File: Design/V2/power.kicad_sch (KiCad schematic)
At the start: 46 parts, among them U1 STM32H747BIT6

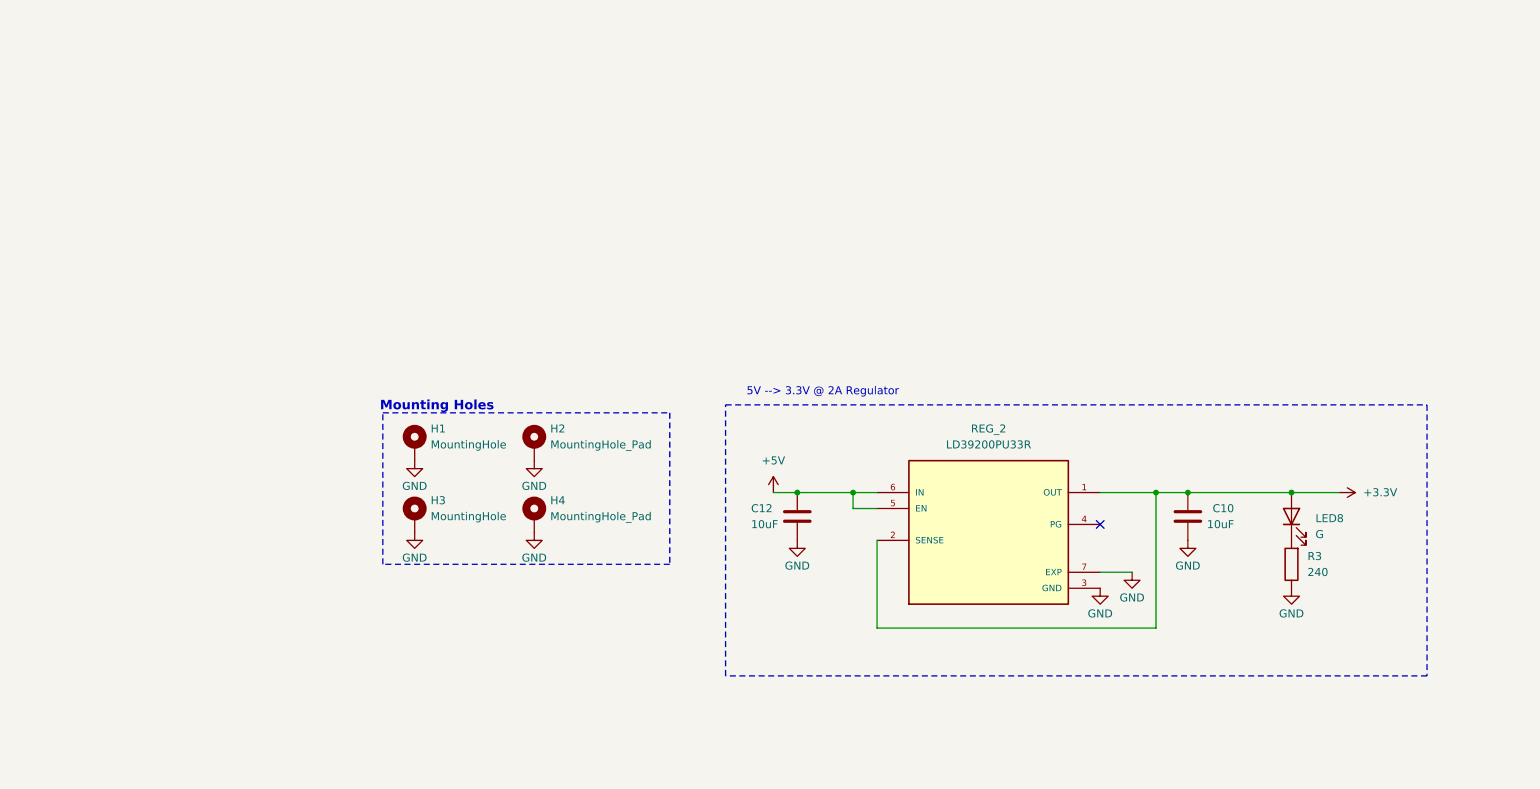
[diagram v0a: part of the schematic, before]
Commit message: power board
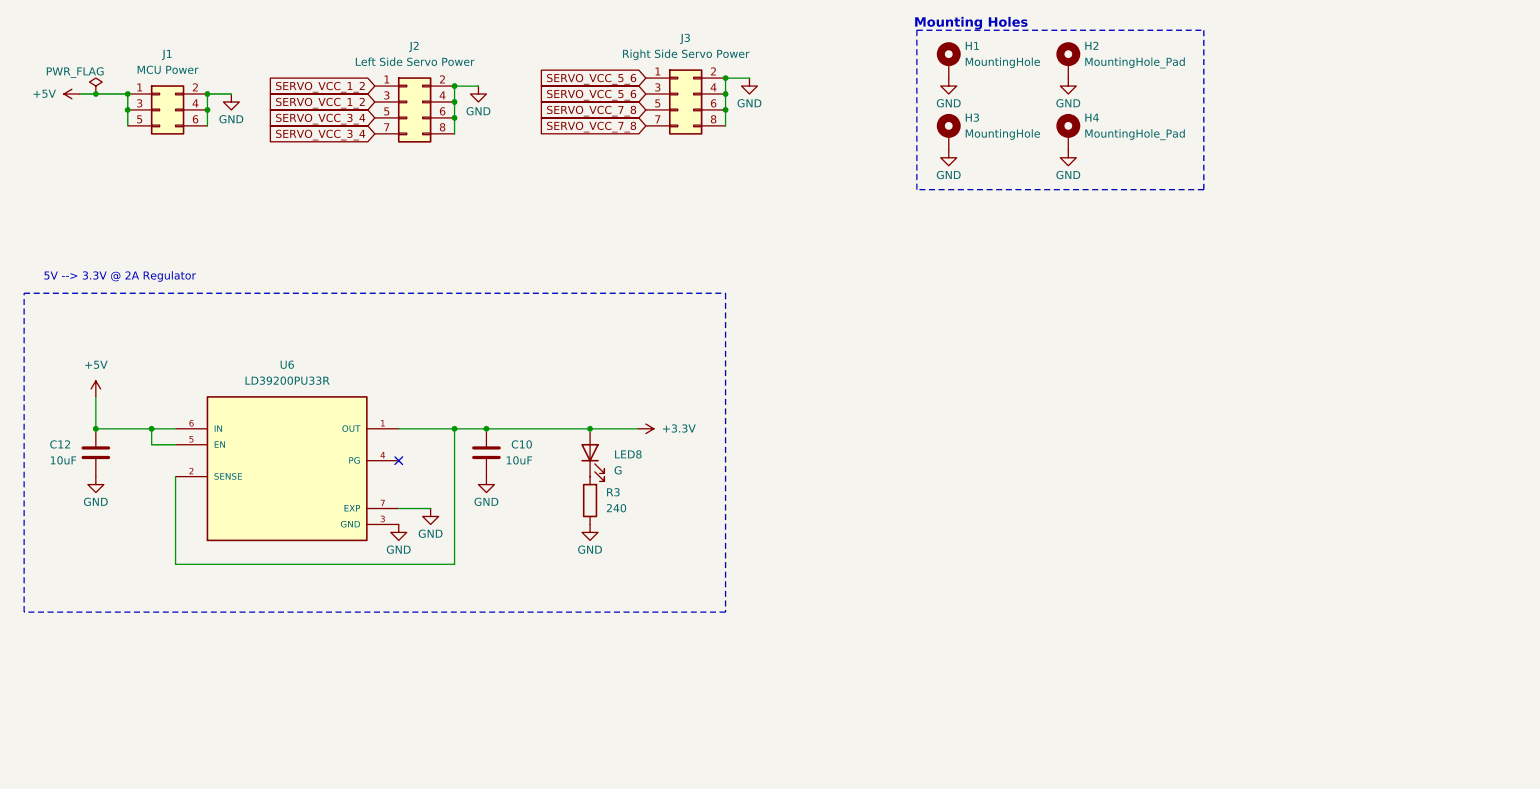
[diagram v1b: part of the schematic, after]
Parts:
- added J1: MCU Power, Connector_PinHeader_2.54mm:PinHeader_2x03_P2.54mm_Vertical, symbol Connector_Generic:Conn_02x03_Odd_Even
- added J2: Left Side Servo Power, Connector_PinHeader_2.54mm:PinHeader_2x04_P2.54mm_Vertical, symbol Connector_Generic:Conn_02x04_Odd_Even
- added J3: Right Side Servo Power, Connector_PinHeader_2.54mm:PinHeader_2x04_P2.54mm_Vertical, symbol Connector_Generic:Conn_02x04_Odd_Even
- renumbered REG_2 to U6
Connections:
- net +5V: now also J1.1 (Pin_1), J1.3 (Pin_3), J1.5 (Pin_5)
- net GND: now also J1.2 (Pin_2), J1.4 (Pin_4), J1.6 (Pin_6), J2.2 (Pin_2), J2.4 (Pin_4), J2.6 (Pin_6), J2.8 (Pin_8), J3.2 (Pin_2), J3.4 (Pin_4), J3.6 (Pin_6), J3.8 (Pin_8)
- new net SERVO_VCC_1_2: J2.1 (Pin_1), J2.3 (Pin_3)
- new net SERVO_VCC_3_4: J2.5 (Pin_5), J2.7 (Pin_7)
- new net SERVO_VCC_5_6: J3.1 (Pin_1), J3.3 (Pin_3)
- new net SERVO_VCC_7_8: J3.5 (Pin_5), J3.7 (Pin_7)
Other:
- moved on the sheet: C10, C12, H1, H2, H3, H4, LED8, R3, U6
